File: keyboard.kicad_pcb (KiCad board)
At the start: 2 copper layers, 12 x 21 mm, 68 parts, among them J1 Conn_01x04_Socket, J3 Conn_01x02_Socket, SW1 SW_Push, SW10 SW_Push, SW11 SW_Push, SW12 SW_Push, SW13 SW_Push, SW14 SW_Push, SW15 SW_Push, SW16 SW_Push, SW17 SW_Push, SW18 SW_Push, SW19 SW_Push, SW2 SW_Push, SW20 SW_Push, SW21 SW_Push, SW22 SW_Push, SW23 SW_Push, SW24 SW_Push, SW25 SW_Push, SW26 SW_Push, SW27 SW_Push, SW28 SW_Push, SW3 SW_Push, SW4 SW_Push, SW401 SW_Push, SW402 SW_Push, SW5 SW_Push, SW6 SW_Push, SW7 SW_Push, SW8 SW_Push, SW9 SW_Push, U1 rp2040-zero

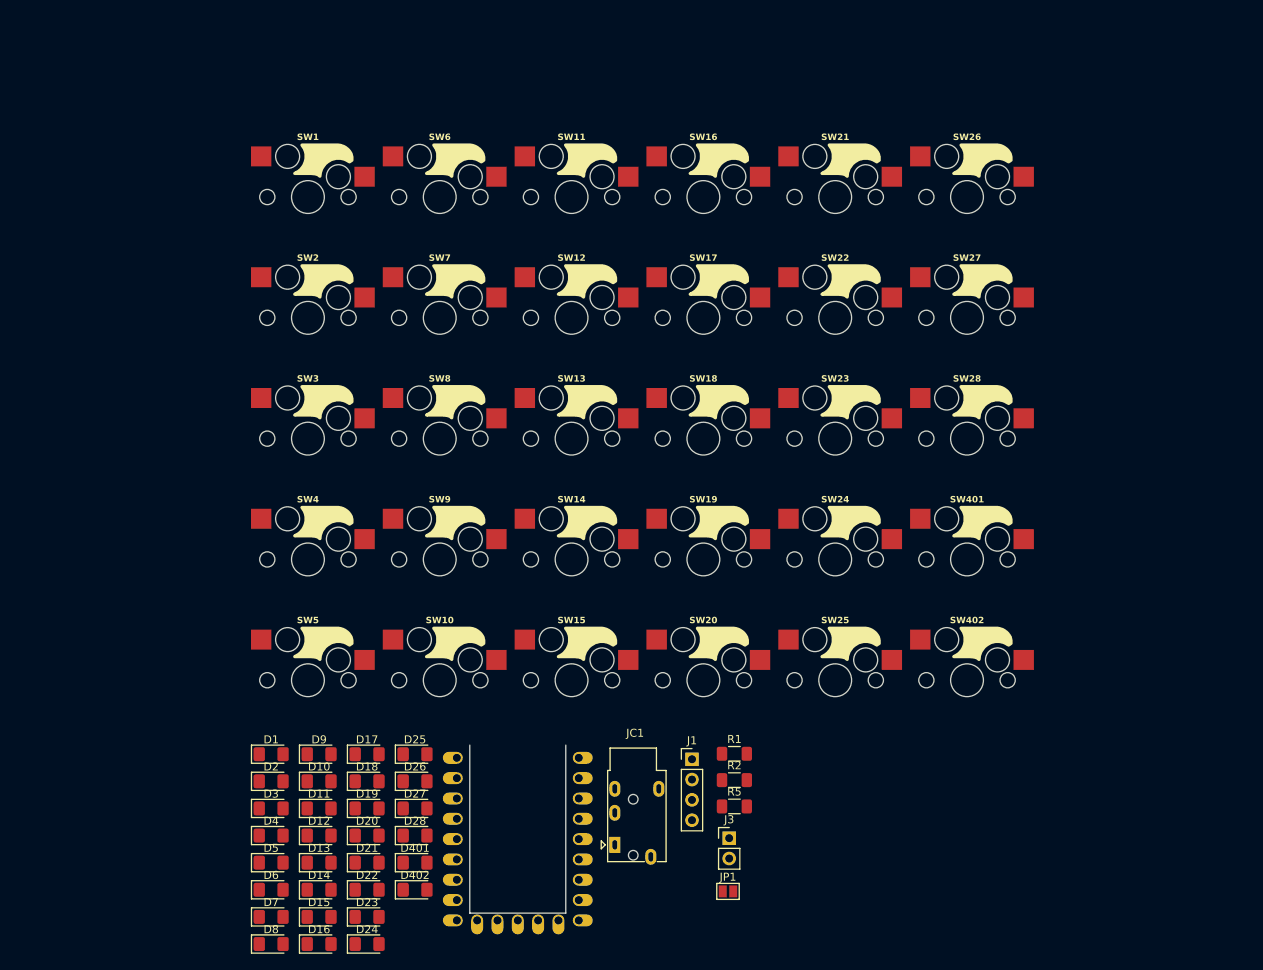
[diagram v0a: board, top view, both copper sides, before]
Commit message: なんとなく形になったので一旦commit
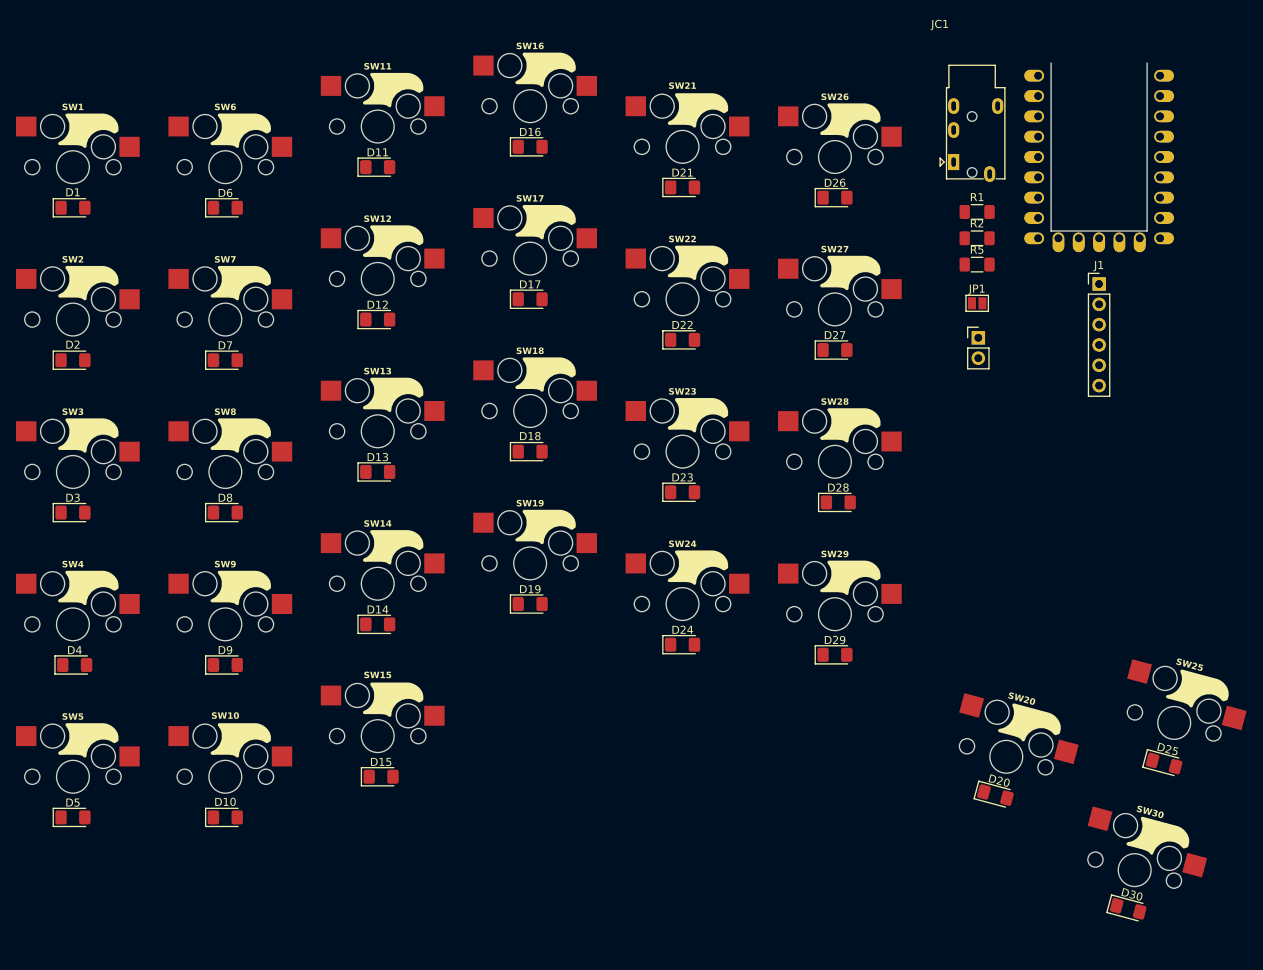
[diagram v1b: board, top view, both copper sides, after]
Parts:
- J1: value Conn_01x04_Socket -> Conn_01x06_Socket; footprint Connector_PinHeader_2.54mm:PinHeader_1x04_P2.54mm_Vertical -> Connector_PinHeader_2.54mm:PinHeader_1x06_P2.54mm_Vertical
- SW5: renamed from SW401; footprint kbd:keyswitch_cherrymx_hotswap_2u -> kbd:keyswitch_cherrymx_hotswap_1u
- moved SW5 115.0 mm to (76.2, 134.0)
- moved U1 112.0 mm to (204.5, 56.5)
- moved D26 110.1 mm to (171.4, 61.6)
- moved D25 101.5 mm to (212.6, 132.3), turned to -15 degrees
- moved D16 99.8 mm to (133.3, 55.2)
- moved JC1 95.3 mm to (186.3, 57.1)
- moved D30 89.6 mm to (208.1, 150.5), turned to -15 degrees
- moved D21 87.1 mm to (152.4, 60.3)
- moved D17 84.8 mm to (133.3, 74.3)
- moved D6 82.1 mm to (95.2, 62.9)
- moved JP1 79.8 mm to (189.2, 74.8)
- moved J1 78.2 mm to (204.5, 72.4)
- moved D11 77.1 mm to (114.3, 57.8)
- moved R1 74.2 mm to (189.2, 63.4)
- moved R2 74.2 mm to (189.2, 66.7)
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- renumbered D9 to D10, D10 to D11, D11 to D12, D12 to D13, D13 to D14, D14 to D15, D15 to D16, D16 to D17, D17 to D18, D18 to D19, D402 to D20, D19 to D21, D20 to D22, D21 to D23, D22 to D24, D23 to D25, D24 to D26, D25 to D27, D26 to D28, D27 to D29, D28 to D30, D401 to D5, D5 to D6, D6 to D7, D7 to D8, D8 to D9, SW9 to SW10, SW10 to SW11, SW11 to SW12, SW12 to SW13, SW13 to SW14, SW14 to SW15, SW15 to SW16, SW16 to SW17, SW17 to SW18, SW18 to SW19, SW402 to SW20, SW19 to SW21, SW20 to SW22, SW21 to SW23, SW22 to SW24, SW23 to SW25, SW24 to SW26, SW25 to SW27, SW26 to SW28, SW27 to SW29, SW28 to SW30, SW5 to SW6, SW6 to SW7, SW7 to SW8, SW8 to SW9
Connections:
- JC1 pad S: Net-(U1-15) -> Net-(J1-Pin_5)
- JC1 pad T: Net-(JP1-A) -> Net-(J1-Pin_6)
- JP1 pad 1: Net-(JP1-A) -> Net-(J1-Pin_6)
- R1 pad 1: Net-(JP1-A) -> Net-(J1-Pin_6)
- R2 pad 1: Net-(JP1-A) -> Net-(J1-Pin_6)
- R5 pad 2: Net-(U1-15) -> Net-(J1-Pin_5)
- U1 pad 16: Net-(U1-15) -> Net-(J1-Pin_5)
- U1 pad 22: Net-(U1-15) -> Net-(J1-Pin_5)
- U1 pad 23: Net-(JP1-A) -> Net-(J1-Pin_6)
